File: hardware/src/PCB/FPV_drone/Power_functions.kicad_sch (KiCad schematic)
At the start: 43 parts, among them IC1 TPS2121RUXT, IC10 AP2112K-3.3TRG1, IC3 USBLC6-2SC6, IC4 AP2112K-3.3TRG1, IC5 DCP3603BCMR - 500kHz, IC8 DCP3603BCMR - 500kHz, J1 TYPE-C-31-M-12

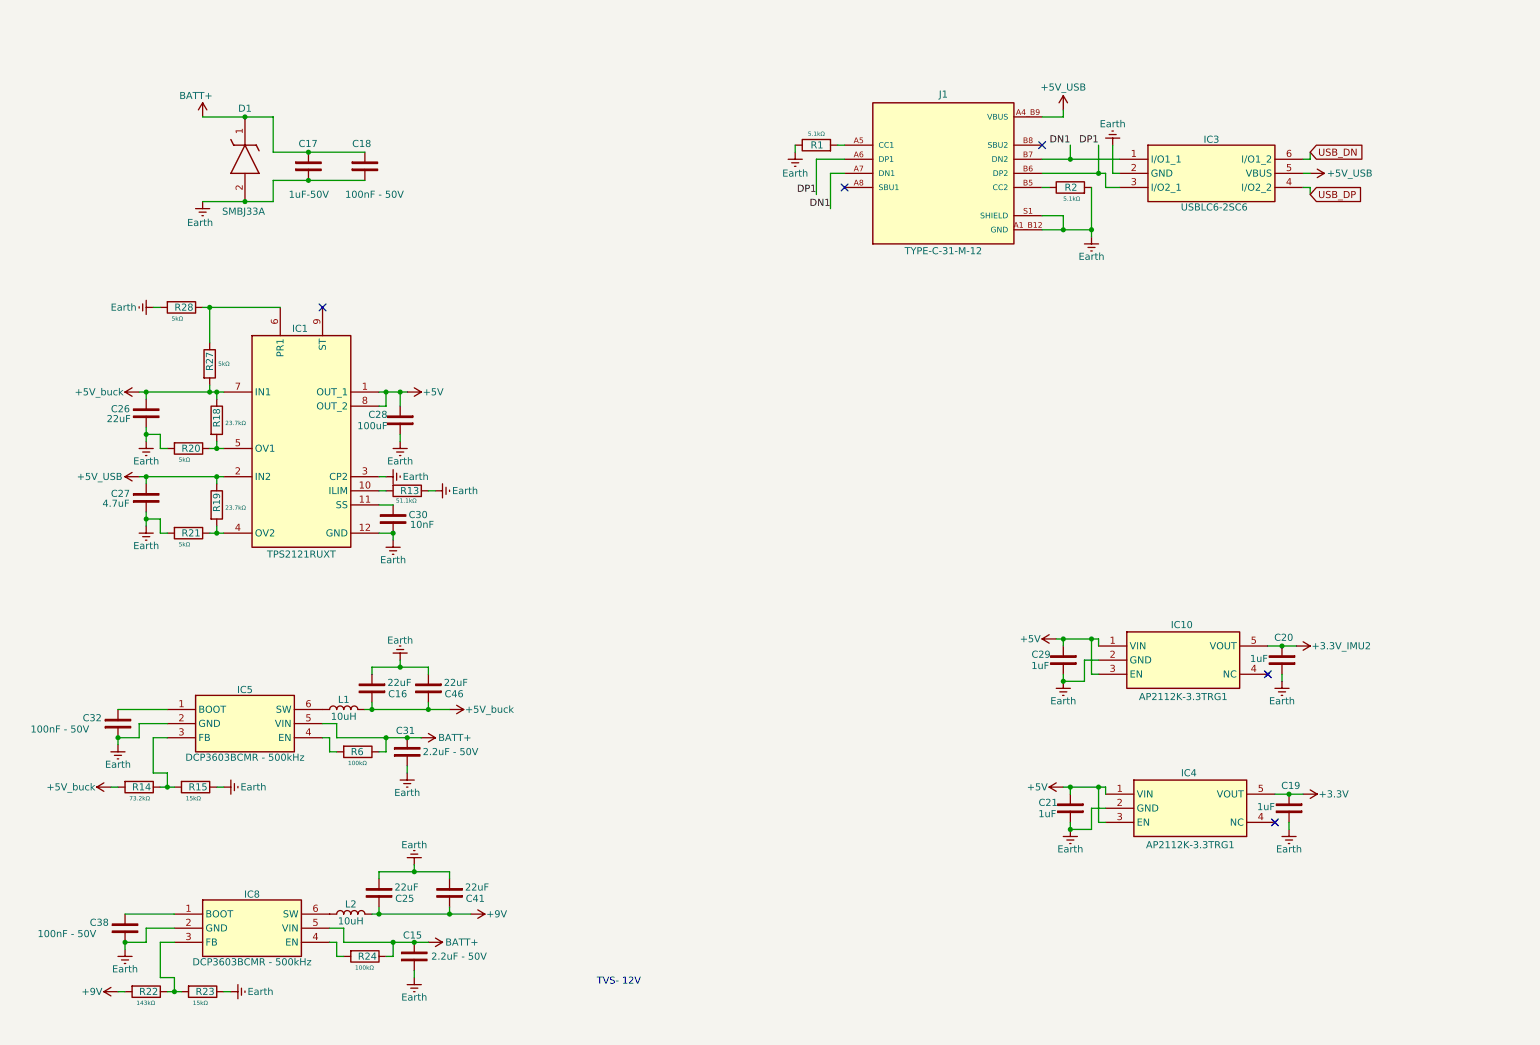
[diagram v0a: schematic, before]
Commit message: Update: schem almost finish
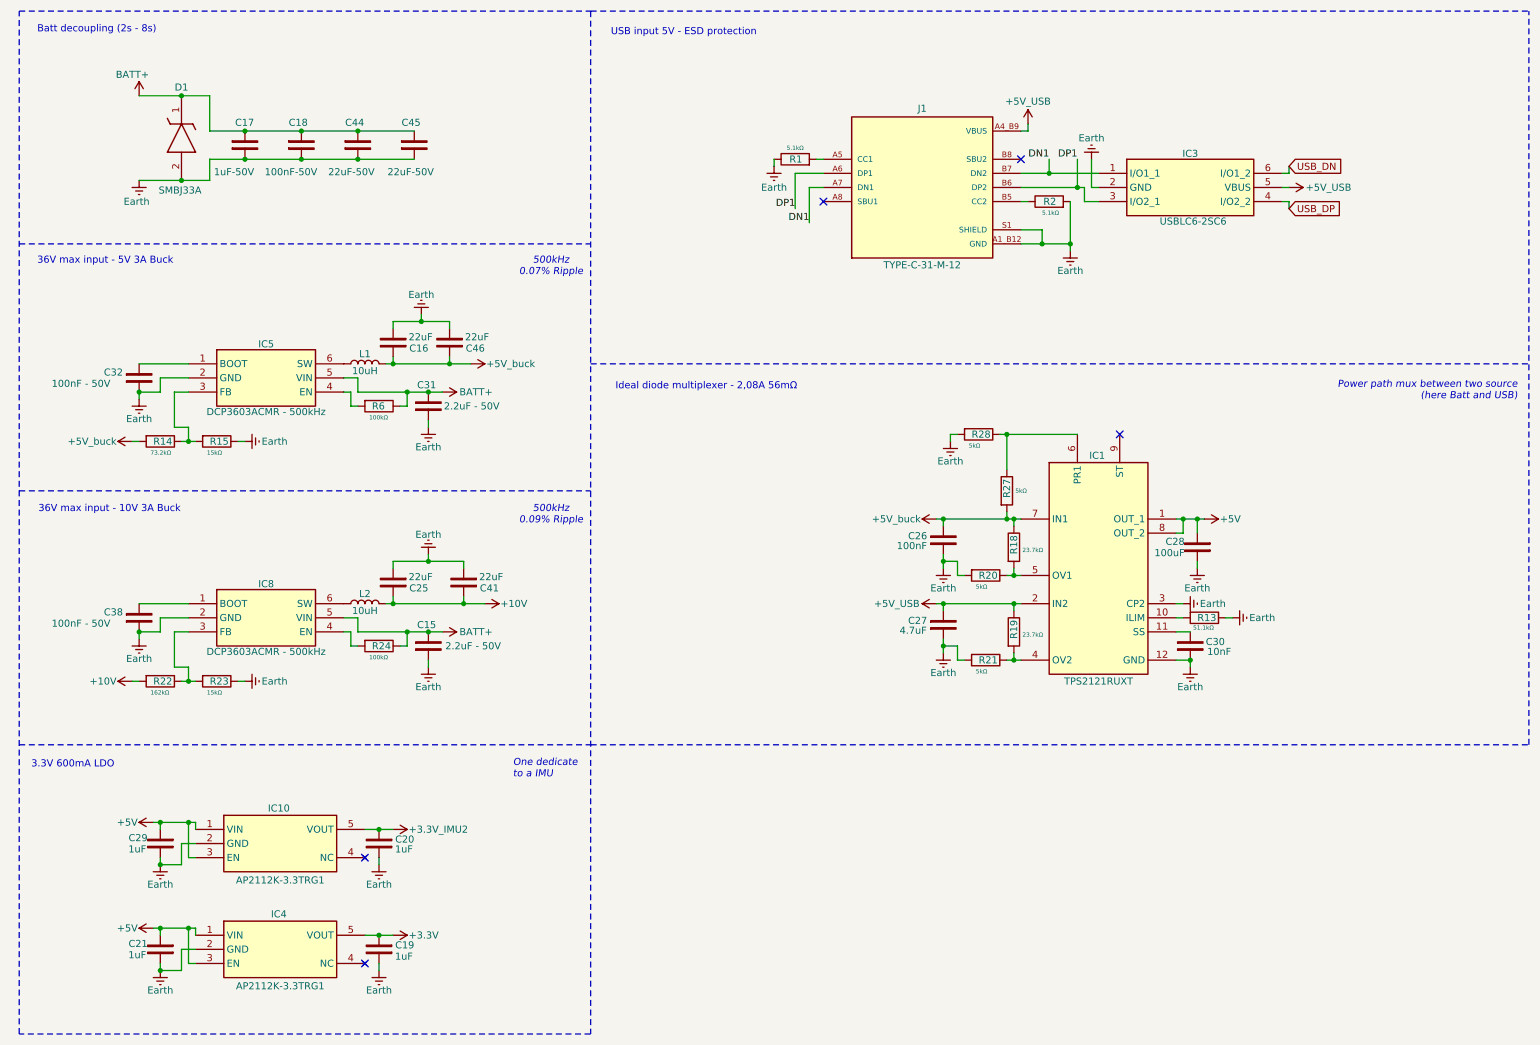
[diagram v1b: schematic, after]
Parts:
- added C44, C45: 22uF-50V, Capacitor_THT:C_Disc_D3.0mm_W2.0mm_P2.50mm, symbol PCM_SL_Devices:Capacitor_NP
- C18: value 100nF - 50V -> 100nF-50V
- C26: value 22uF -> 100nF
- IC5, IC8: value DCP3603BCMR - 500kHz -> DCP3603ACMR - 500kHz
- R22: value 143kΩ -> 162kΩ
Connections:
- net BATT+: now also C44.1, C45.1
- net Earth: now also C44.2, C45.2
- net +9V renamed +10V
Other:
- note added: "3.3V 600mA LDO"
- note added: "36V max input - 10V 3A Buck"
- note added: "36V max input - 5V 3A Buck"
- note added: "500kHz 0.07% Ripple"
- note added: "500kHz 0.09% Ripple"
- note added: "Batt decoupling (2s - 8s)"
- note added: "Ideal diode multiplexer - 2,08A 56mΩ"
- note added: "One dedicate to a IMU"
- note added: "Power path mux between two source (here Batt and USB)"
- note added: "USB input 5V - ESD protection"
- note removed: "TVS- 12V"
- moved on the sheet: C15, C16, C17, C18, C19, C20, C21, C25, C26, C27, C28, C29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
